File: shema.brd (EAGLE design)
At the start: 100 x 80 mm, 20 parts

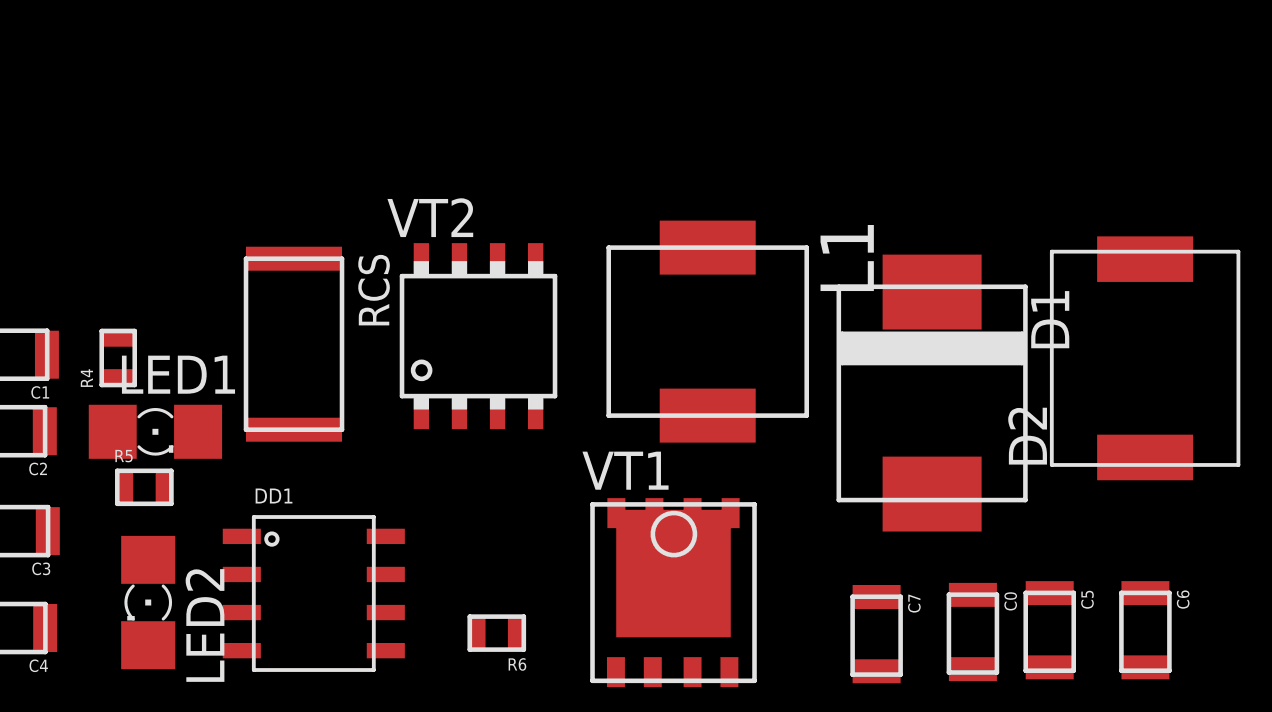
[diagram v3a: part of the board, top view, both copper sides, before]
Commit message: файлы изменения
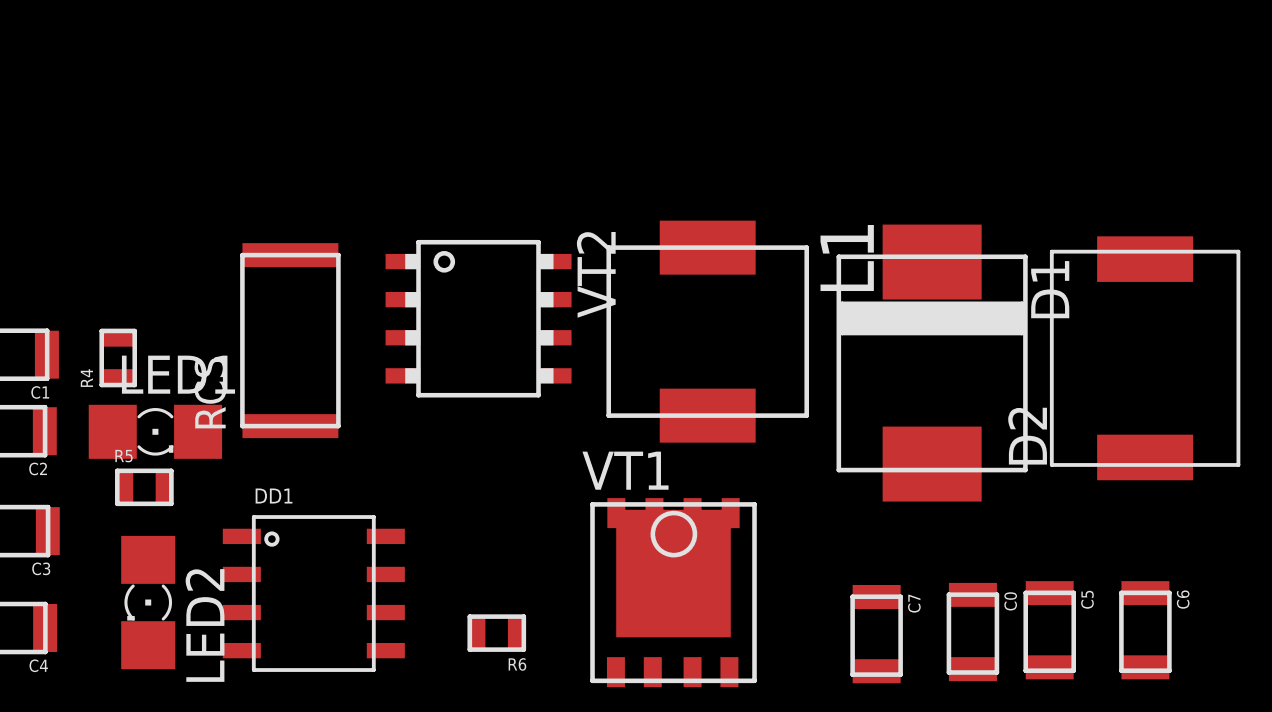
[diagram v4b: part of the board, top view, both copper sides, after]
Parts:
- moved D1 1.00 mm to (33.8, 19.8)
- moved VT2 0.58 mm to (18.7, 21.3), turned to 270 degrees
- moved RCS 0.17 mm to (12.4, 20.6), turned to 90 degrees
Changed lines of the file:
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@@
 <attribute name="VALUE" x="30.657" y="12.3" size="0.4064" layer="27" rot="R270"/>
 </element>
-<element name="D1" library="1_DIOD" package="CB417-15" value="B560C-13-F" x="33.83" y="18.8" smashed="yes" rot="R270">
-<attribute name="NAME" x="37.132" y="22.356" size="1.27" layer="25" rot="R270"/>
-<attribute name="VALUE" x="29.258" y="22.229" size="1.27" layer="27" rot="R270"/>
+<element name="D1" library="1_DIOD" package="CB417-15" value="B560C-13-F" x="33.83" y="19.8" smashed="yes" rot="R270">
+<attribute name="NAME" x="37.132" y="23.356" size="1.27" layer="25" rot="R270"/>
+<attribute name="VALUE" x="29.258" y="23.229" size="1.27" layer="27" rot="R270"/>
 </element>
 <element name="D2" library="1_DIOD" package="DIOD" value="SS36C" x="40.93" y="19.97" smashed="yes" rot="R90">
@@
 <attribute name="VALUE" x="20.327" y="11.937" size="0.4064" layer="27" rot="R180"/>
 </element>
-<element name="RCS" library="1_RESISTOR" package="2512" value="0.015" x="12.56" y="20.44" smashed="yes" rot="R270">
-<attribute name="NAME" x="14.719" y="23.488" size="1.016" layer="25" rot="R270"/>
-<attribute name="VALUE" x="9.766" y="23.615" size="1.016" layer="27" rot="R270"/>
+<element name="RCS" library="1_RESISTOR" package="2512" value="0.015" x="12.44" y="20.56" smashed="yes" rot="R90">
+<attribute name="NAME" x="10.281" y="17.512" size="1.016" layer="25" rot="R90"/>
+<attribute name="VALUE" x="15.234" y="17.385" size="1.016" layer="27" rot="R90"/>
 </element>
 <element name="VT1" library="1_TRANSISTOR (2)" package="PDFN5*6-8L" value="TRANSISTORN" x="25.21" y="12.16" smashed="yes">
@@
 <attribute name="VALUE" x="22.285" y="10.162" size="1.27" layer="27" rot="R90"/>
 </element>
-<element name="VT2" library="1_TRANSISTOR (2)" package="SOP-8" value="TRAN_P" x="18.71" y="20.71" smashed="yes">
-<attribute name="NAME" x="15.662" y="24.012" size="1.27" layer="25"/>
-<attribute name="VALUE" x="15.535" y="16.265" size="1.27" layer="27"/>
+<element name="VT2" library="1_TRANSISTOR (2)" package="SOP-8" value="TRAN_P" x="18.71" y="21.29" smashed="yes" rot="R270">
+<attribute name="NAME" x="22.012" y="24.338" size="1.27" layer="25" rot="R270"/>
+<attribute name="VALUE" x="14.265" y="24.465" size="1.27" layer="27" rot="R270"/>
 </element>
 </elements>
@@
 <contactref element="R4" pad="P$2"/>
 <wire x1="10.82" y1="12.765" x2="15.62" y2="12.765" width="0" layer="19" extent="1-1"/>
-<wire x1="12.56" y1="17.59" x2="10.82" y2="12.765" width="0" layer="19" extent="1-1"/>
-<wire x1="6.7" y1="20.658" x2="12.56" y2="17.59" width="0" layer="19" extent="1-1"/>
+<wire x1="12.44" y1="23.41" x2="10.82" y2="12.765" width="0" layer="19" extent="1-1"/>
+<wire x1="6.7" y1="20.658" x2="12.44" y2="23.41" width="0" layer="19" extent="1-1"/>
 <wire x1="4.324" y1="20.09" x2="6.7" y2="20.658" width="0" layer="19" extent="1-1"/>
 <wire x1="4.254" y1="17.54" x2="4.324" y2="20.09" width="0" layer="19" extent="1-1"/>
@@
 <contactref element="VT2" pad="P$8"/>
 <wire x1="26.35" y1="23.66" x2="40.93" y2="23.275" width="0" layer="19" extent="1-1"/>
-<wire x1="20.615" y1="18.11" x2="26.35" y2="23.66" width="0" layer="19" extent="1-1"/>
-<wire x1="19.345" y1="18.11" x2="20.615" y2="18.11" width="0" layer="19" extent="1-1"/>
-<wire x1="18.075" y1="18.11" x2="19.345" y2="18.11" width="0" layer="19" extent="1-1"/>
-<wire x1="16.805" y1="18.11" x2="18.075" y2="18.11" width="0" layer="19" extent="1-1"/>
+<wire x1="16.11" y1="19.385" x2="26.35" y2="23.66" width="0" layer="19" extent="1-1"/>
+<wire x1="16.11" y1="20.655" x2="16.11" y2="19.385" width="0" layer="19" extent="1-1"/>
+<wire x1="16.11" y1="21.925" x2="16.11" y2="20.655" width="0" layer="19" extent="1-1"/>
+<wire x1="16.11" y1="23.195" x2="16.11" y2="21.925" width="0" layer="19" extent="1-1"/>
 </signal>
 <signal name="N$6">
@@
 <contactref element="VT1" pad="P$4"/>
 <contactref element="VT1" pad="P$9"/>
-<wire x1="26.35" y1="18.06" x2="33.83" y2="22.179" width="0" layer="19" extent="1-1"/>
+<wire x1="26.35" y1="18.06" x2="33.83" y2="23.179" width="0" layer="19" extent="1-1"/>
 <wire x1="25.845" y1="14.81" x2="26.35" y2="18.06" width="0" layer="19" extent="1-1"/>
 <wire x1="27.115" y1="14.81" x2="25.845" y2="14.81" width="0" layer="19" extent="1-1"/>
@@
 <contactref element="DD1" pad="6"/>
 <contactref element="VT2" pad="P$4"/>
-<wire x1="15.62" y1="11.495" x2="20.615" y2="23.31" width="0" layer="19" extent="1-1"/>
+<wire x1="15.62" y1="11.495" x2="21.31" y2="19.385" width="0" layer="19" extent="1-1"/>
 </signal>
 <signal name="N$1">
@@
 <wire x1="35.19" y1="12.084" x2="37.75" y2="12.144" width="0" layer="19" extent="1-1"/>
 <wire x1="31.98" y1="12.014" x2="35.19" y2="12.084" width="0" layer="19" extent="1-1"/>
-<wire x1="33.83" y1="15.445" x2="35.19" y2="12.084" width="0" layer="19" extent="1-1"/>
+<wire x1="33.83" y1="16.445" x2="35.19" y2="12.084" width="0" layer="19" extent="1-1"/>
 <wire x1="10.82" y1="11.495" x2="31.98" y2="12.014" width="0" layer="19" extent="1-1"/>
 </signal>
@@
 <contactref element="VT2" pad="P$2"/>
 <contactref element="VT2" pad="P$3"/>
-<wire x1="19.345" y1="23.31" x2="18.075" y2="23.31" width="0" layer="19" extent="1-1"/>
-<wire x1="16.805" y1="23.31" x2="18.075" y2="23.31" width="0" layer="19" extent="1-1"/>
-<wire x1="12.56" y1="23.29" x2="16.805" y2="23.31" width="0" layer="19" extent="1-1"/>
-<wire x1="15.62" y1="14.035" x2="16.805" y2="23.31" width="0" layer="19" extent="1-1"/>
+<wire x1="21.31" y1="20.655" x2="21.31" y2="21.925" width="0" layer="19" extent="1-1"/>
+<wire x1="21.31" y1="23.195" x2="21.31" y2="21.925" width="0" layer="19" extent="1-1"/>
+<wire x1="12.44" y1="17.71" x2="21.31" y2="23.195" width="0" layer="19" extent="1-1"/>
+<wire x1="15.62" y1="14.035" x2="21.31" y2="23.195" width="0" layer="19" extent="1-1"/>
 </signal>
 </signals>

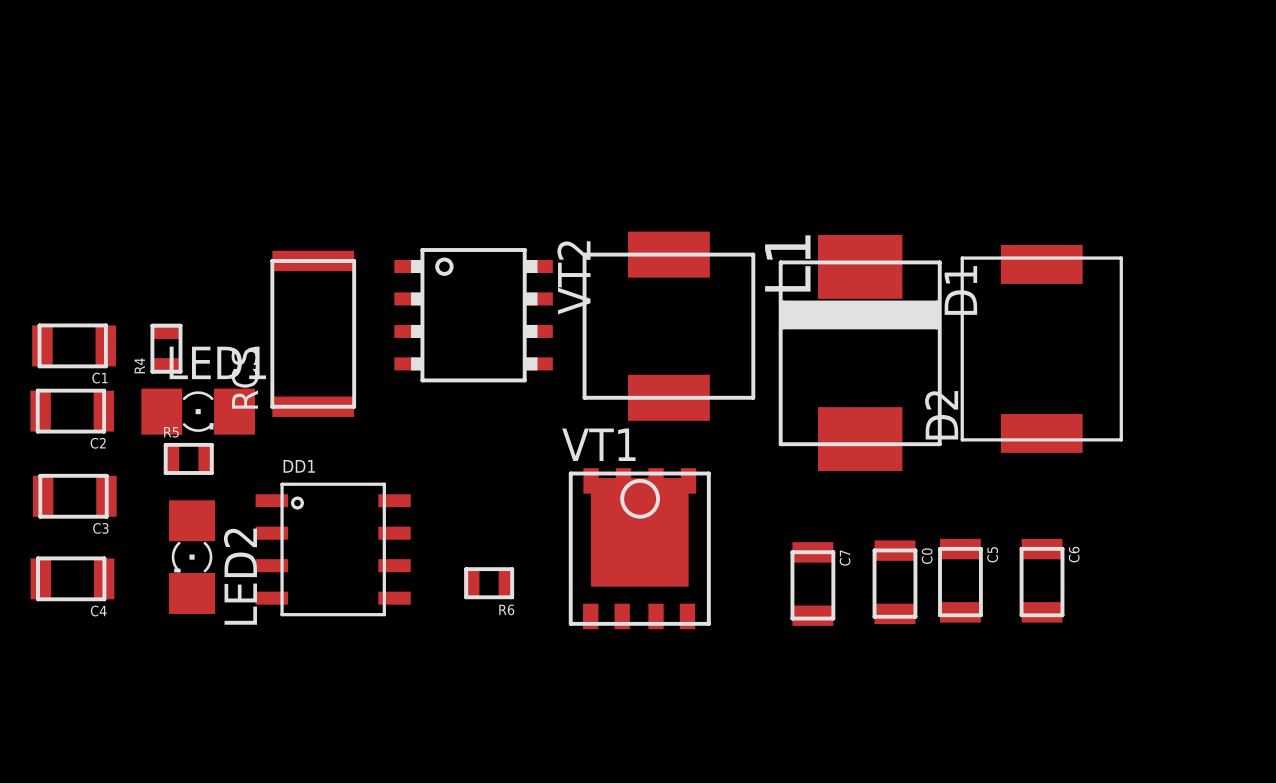
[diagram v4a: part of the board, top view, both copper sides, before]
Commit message: файлы изменения
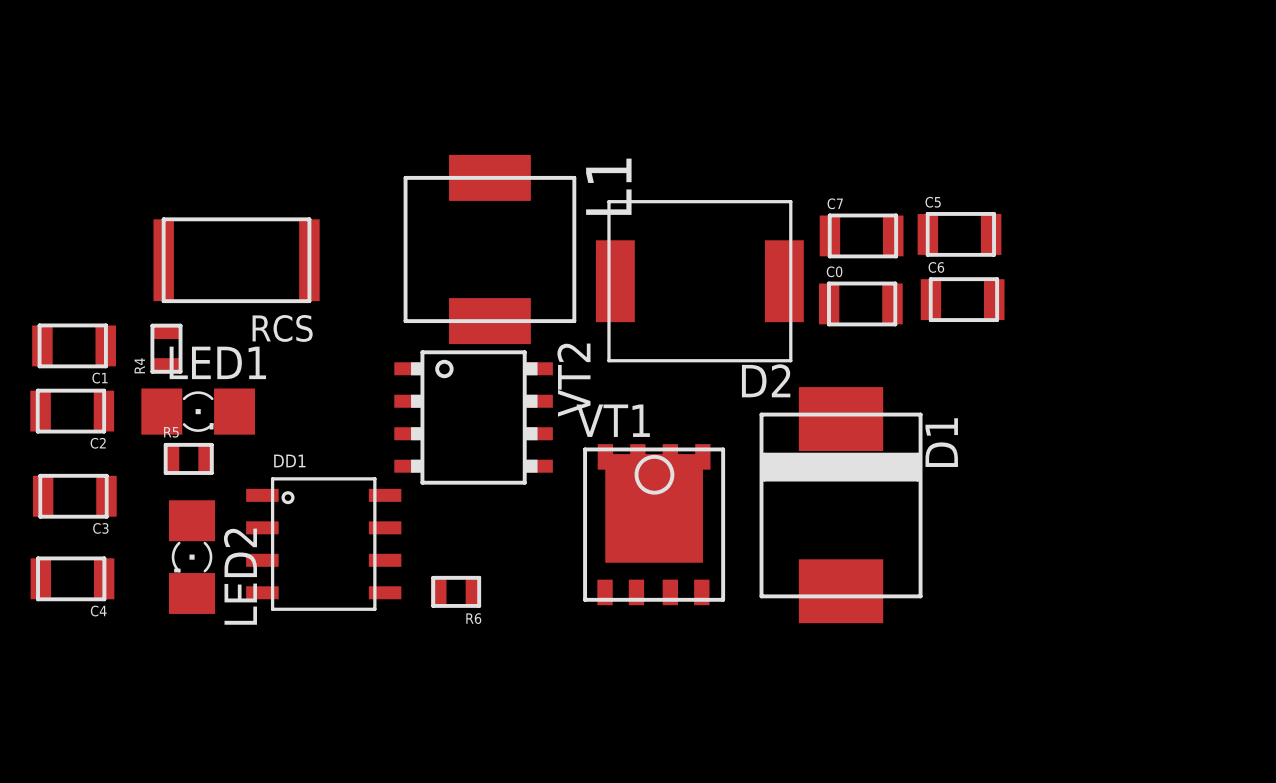
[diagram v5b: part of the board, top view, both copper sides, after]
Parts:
- moved C7 13.7 mm to (33.9, 24.4), turned to 0 degrees
- moved D2 13.6 mm to (27.6, 22.6), turned to 180 degrees
- moved C5 13.5 mm to (37.7, 24.4), turned to 0 degrees
- moved C6 11.4 mm to (37.8, 21.9), turned to 0 degrees
- moved C0 11.0 mm to (33.9, 21.7), turned to 0 degrees
- moved L1 7.62 mm to (19.4, 23.9)
- moved D1 6.00 mm to (33.1, 13.8)
- moved RCS 4.16 mm to (9.44, 23.4), turned to 180 degrees
- moved VT2 4.00 mm to (18.7, 17.3)
- moved R6 1.33 mm to (18.0, 10.5)
- moved VT1 1.09 mm to (25.8, 13.1)
- moved DD1 0.43 mm to (12.8, 12.3)
